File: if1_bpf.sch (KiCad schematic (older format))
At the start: 8 parts

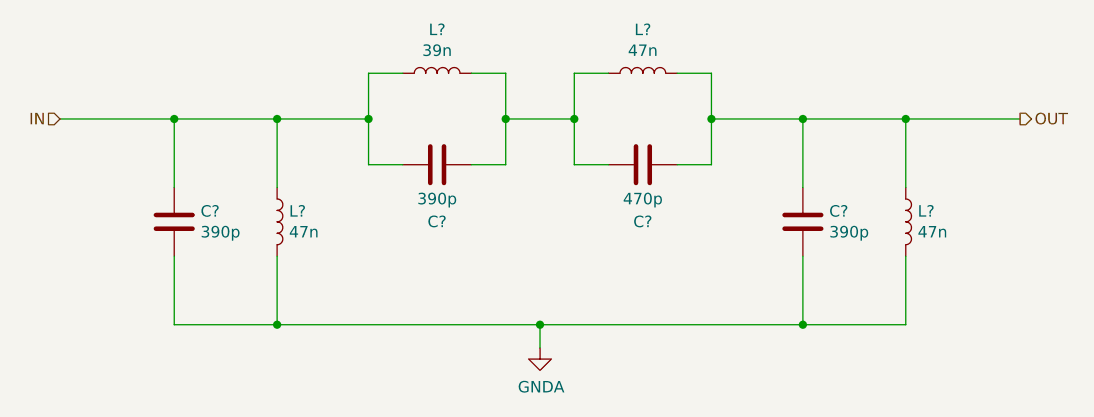
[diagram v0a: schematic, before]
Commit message: PCB is Done... Needs DRC check
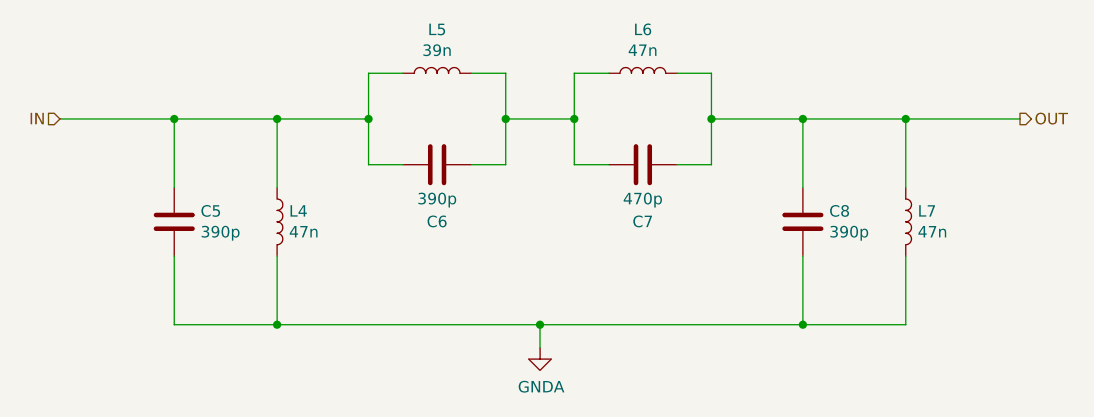
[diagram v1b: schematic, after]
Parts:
- gave numbers to parts that had none: 8
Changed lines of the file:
@@
 $Descr A4 11693 8268
 encoding utf-8
-Sheet 4 14
+Sheet 4 7
 Title "37,224 MHz Bandpass filter"
 Date "2021 january"
@@
 OUT
 $Comp
-L Device:C C?
+L Device:C C5
 U 1 1 600431FC
 P 4450 3850
-F 0 "C?" H 4565 3896 50  0000 L CNN
+F 0 "C5" H 4565 3896 50  0000 L CNN
 F 1 "390p" H 4565 3805 50  0000 L CNN
 F 2 "Capacitor_SMD:C_0805_2012Metric_Pad1.18x1.45mm_HandSolder" H 4488 3700 50  0001 C CNN
@@
 $EndComp
 $Comp
-L Device:L L?
+L Device:L L4
 U 1 1 600436A2
 P 4900 3850
-F 0 "L?" H 4952 3896 50  0000 L CNN
+F 0 "L4" H 4952 3896 50  0000 L CNN
 F 1 "47n" H 4952 3805 50  0000 L CNN
 F 2 "Inductor_SMD:L_0603_1608Metric_Pad1.05x0.95mm_HandSolder" H 4900 3850 50  0001 C CNN
@@
 $EndComp
 $Comp
-L Device:L L?
+L Device:L L5
 U 1 1 600471E0
 P 5600 3200
-F 0 "L?" V 5790 3200 50  0000 C CNN
+F 0 "L5" V 5790 3200 50  0000 C CNN
 F 1 "39n" V 5699 3200 50  0000 C CNN
 F 2 "Inductor_SMD:L_0402_1005Metric_Pad0.77x0.64mm_HandSolder" H 5600 3200 50  0001 C CNN
@@
 $EndComp
 $Comp
-L Device:C C?
+L Device:C C6
 U 1 1 6004779D
 P 5600 3600
-F 0 "C?" V 5350 3600 50  0000 C CNN
+F 0 "C6" V 5350 3600 50  0000 C CNN
 F 1 "390p" V 5450 3600 50  0000 C CNN
 F 2 "Capacitor_SMD:C_0805_2012Metric_Pad1.18x1.45mm_HandSolder" H 5638 3450 50  0001 C CNN
@@
 $EndComp
 $Comp
-L Device:L L?
+L Device:L L6
 U 1 1 6004D573
 P 6500 3200
-F 0 "L?" V 6690 3200 50  0000 C CNN
+F 0 "L6" V 6690 3200 50  0000 C CNN
 F 1 "47n" V 6599 3200 50  0000 C CNN
 F 2 "Inductor_SMD:L_0603_1608Metric_Pad1.05x0.95mm_HandSolder" H 6500 3200 50  0001 C CNN
@@
 $EndComp
 $Comp
-L Device:C C?
+L Device:C C7
 U 1 1 6004D579
 P 6500 3600
-F 0 "C?" V 6250 3600 50  0000 C CNN
+F 0 "C7" V 6250 3600 50  0000 C CNN
 F 1 "470p" V 6350 3600 50  0000 C CNN
 F 2 "Capacitor_SMD:C_0805_2012Metric_Pad1.18x1.45mm_HandSolder" H 6538 3450 50  0001 C CNN
@@
 $EndComp
 $Comp
-L Device:C C?
+L Device:C C8
 U 1 1 6004E74D
 P 7200 3850
-F 0 "C?" H 7315 3896 50  0000 L CNN
+F 0 "C8" H 7315 3896 50  0000 L CNN
 F 1 "390p" H 7315 3805 50  0000 L CNN
 F 2 "Capacitor_SMD:C_0805_2012Metric_Pad1.18x1.45mm_HandSolder" H 7238 3700 50  0001 C CNN
@@
 $EndComp
 $Comp
-L Device:L L?
+L Device:L L7
 U 1 1 6004E753
 P 7650 3850
-F 0 "L?" H 7702 3896 50  0000 L CNN
+F 0 "L7" H 7702 3896 50  0000 L CNN
 F 1 "47n" H 7702 3805 50  0000 L CNN
 F 2 "Inductor_SMD:L_0603_1608Metric_Pad1.05x0.95mm_HandSolder" H 7650 3850 50  0001 C CNN
@@
 	6050 4300 7200 4300
 $Comp
-L power:GNDA #PWR?
+L power:GNDA #PWR06
 U 1 1 60071173
 P 6050 4400
-F 0 "#PWR?" H 6050 4150 50  0001 C CNN
+F 0 "#PWR06" H 6050 4150 50  0001 C CNN
 F 1 "GNDA" H 6055 4227 50  0000 C CNN
 F 2 "" H 6050 4400 50  0001 C CNN
